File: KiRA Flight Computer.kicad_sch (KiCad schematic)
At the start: 44 parts, among them J1 Conn_01x04_Pin, J2 USB_C_Receptacle_USB2.0_14P, SW1 SW_Push, SW2 SW_SPDT, U1 ICM-426788P, U2 STM32F407VGTx, U3 MMC5883MA, U4 DPS368, U6 Wio-SX1262, U7 USBLC6-2P6, Y1 16MHz 7pF, Y2 OV_7604

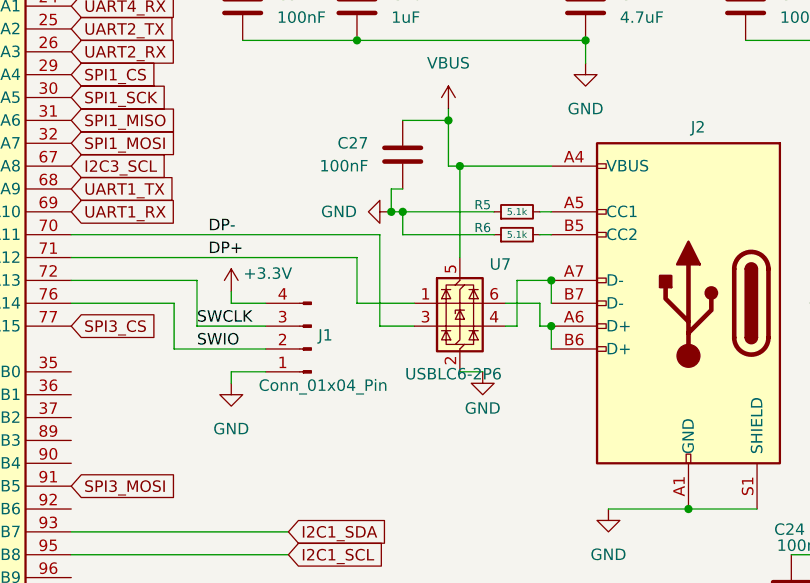
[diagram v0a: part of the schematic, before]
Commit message: Update PCB
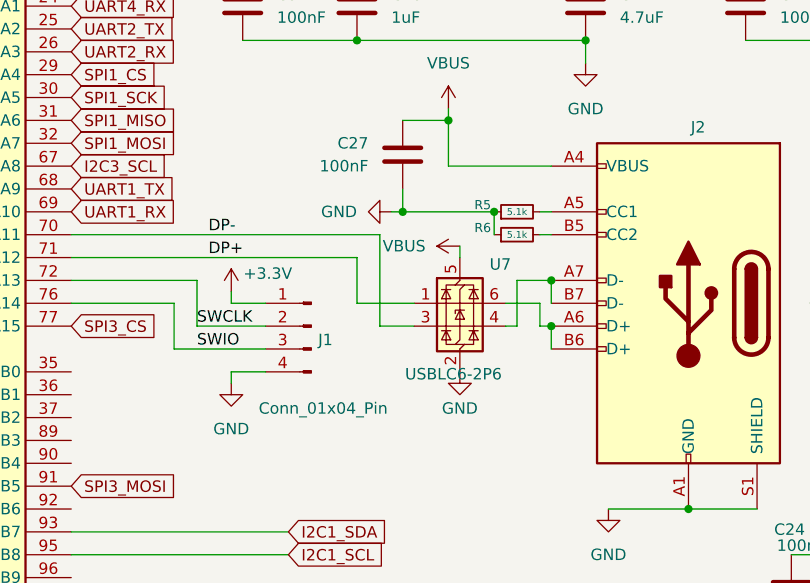
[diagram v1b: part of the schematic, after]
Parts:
- SW1: footprint Button_Switch_SMD:SW_Push_1P1T_NO_CK_PTS125Sx43PSMTR -> Button_Switch_SMD:SW_Push_1P1T_NO_CK_KSC6xxJ
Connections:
- net +3.3V: now also J1.1 (Pin_1); no longer J1.4 (Pin_4)
- net GND: now also J1.4 (Pin_4); no longer J1.1 (Pin_1)
- net SWCLK: now also J1.2 (Pin_2); no longer J1.3 (Pin_3)
- net SWIO: now also J1.3 (Pin_3); no longer J1.2 (Pin_2)
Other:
- moved on the sheet: J1
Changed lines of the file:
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@@
 	(paper "A4")
 	(junction
-		(at 135.89 63.5)
+		(at 217.17 48.26)
 		(diameter 0)
 		(color 0 0 0 0)
 	)
 	(junction
-		(at 217.17 48.26)
+		(at 135.89 63.5)
 		(diameter 0)
 		(color 0 0 0 0)
@@
 	)
 	(junction
+		(at 146.05 63.5)
+		(diameter 0)
+		(color 0 0 0 0)
+	)
+	(junction
 		(at 143.51 27.94)
 		(diameter 0)
@@
 	)
 	(junction
-		(at 134.62 63.5)
-		(diameter 0)
-		(color 0 0 0 0)
-	)
-	(junction
 		(at 16.51 77.47)
 		(diameter 0)
@@
 	)
 	(junction
-		(at 142.24 58.42)
-		(diameter 0)
-		(color 0 0 0 0)
-	)
-	(junction
 		(at 212.09 105.41)
 		(diameter 0)
@@
 	(wire
 		(pts
-			(xy 142.24 81.28) (xy 144.78 81.28)
-		)
-		(stroke
-			(width 0)
-			(type default)
-		)
-	)
-	(wire
-		(pts
 			(xy 156.21 20.32) (xy 168.91 20.32)
 		)
@@
 	(wire
 		(pts
-			(xy 135.89 66.04) (xy 135.89 63.5)
+			(xy 146.05 66.04) (xy 146.05 63.5)
 		)
 		(stroke
@@
 	(wire
 		(pts
-			(xy 146.05 66.04) (xy 135.89 66.04)
-		)
-		(stroke
-			(width 0)
-			(type default)
-		)
-	)
-	(wire
-		(pts
 			(xy 195.58 101.6) (xy 195.58 106.68)
 		)
@@
 	(wire
 		(pts
-			(xy 134.62 63.5) (xy 135.89 63.5)
-		)
-		(stroke
-			(width 0)
-			(type default)
-		)
-	)
-	(wire
-		(pts
 			(xy 259.08 128.27) (xy 259.08 134.62)
 		)
@@
 	(wire
 		(pts
+			(xy 135.89 63.5) (xy 146.05 63.5)
+		)
+		(stroke
+			(width 0)
+			(type default)
+		)
+	)
+	(wire
+		(pts
 			(xy 78.74 25.4) (xy 78.74 27.94)
 		)
@@
 	(wire
 		(pts
-			(xy 135.89 60.96) (xy 134.62 60.96)
-		)
-		(stroke
-			(width 0)
-			(type default)
-		)
-	)
-	(wire
-		(pts
-			(xy 142.24 58.42) (xy 152.4 58.42)
-		)
-		(stroke
-			(width 0)
-			(type default)
-		)
-	)
-	(wire
-		(pts
 			(xy 99.06 68.58) (xy 130.81 68.58)
 		)
@@
 	(wire
 		(pts
-			(xy 140.97 58.42) (xy 142.24 58.42)
+			(xy 140.97 58.42) (xy 152.4 58.42)
 		)
 		(stroke
@@
 	(wire
 		(pts
-			(xy 193.04 109.22) (xy 193.04 106.68)
+			(xy 135.89 63.5) (xy 134.62 63.5)
 		)
 		(stroke
@@
 	(wire
 		(pts
-			(xy 135.89 132.08) (xy 133.35 132.08)
+			(xy 193.04 109.22) (xy 193.04 106.68)
 		)
 		(stroke
@@
 	(wire
 		(pts
-			(xy 19.05 35.56) (xy 19.05 38.1)
+			(xy 135.89 132.08) (xy 133.35 132.08)
 		)
 		(stroke
@@
 	(wire
 		(pts
-			(xy 21.59 71.12) (xy 21.59 85.09)
+			(xy 19.05 35.56) (xy 19.05 38.1)
 		)
 		(stroke
@@
 	(wire
 		(pts
-			(xy 130.81 20.32) (xy 143.51 20.32)
+			(xy 21.59 71.12) (xy 21.59 85.09)
 		)
 		(stroke
@@
 	(wire
 		(pts
-			(xy 38.1 77.47) (xy 31.75 77.47)
+			(xy 130.81 20.32) (xy 143.51 20.32)
 		)
 		(stroke
@@
 	(wire
 		(pts
-			(xy 156.21 35.56) (xy 156.21 36.83)
+			(xy 38.1 77.47) (xy 31.75 77.47)
 		)
 		(stroke
@@
 	(wire
 		(pts
-			(xy 219.71 127) (xy 212.09 127)
+			(xy 156.21 35.56) (xy 156.21 36.83)
 		)
 		(stroke
@@
 	(wire
 		(pts
-			(xy 135.89 63.5) (xy 146.05 63.5)
+			(xy 219.71 127) (xy 212.09 127)
 		)
 		(stroke
@@
 	(wire
 		(pts
-			(xy 142.24 58.42) (xy 142.24 68.58)
-		)
-		(stroke
-			(width 0)
-			(type default)
-		)
-	)
-	(wire
-		(pts
 			(xy 133.35 66.04) (xy 133.35 76.2)
 		)
@@
 	(wire
 		(pts
-			(xy 134.62 60.96) (xy 134.62 63.5)
+			(xy 135.89 60.96) (xy 135.89 63.5)
 		)
 		(stroke
@@
 	(wire
 		(pts
+			(xy 142.24 67.31) (xy 142.24 68.58)
+		)
+		(stroke
+			(width 0)
+			(type default)
+		)
+	)
+	(wire
+		(pts
 			(xy 71.12 25.4) (xy 71.12 27.94)
 		)
@@
 			)
 		)
-		(property "Footprint" "Button_Switch_SMD:SW_Push_1P1T_NO_CK_PTS125Sx43PSMTR"
+		(property "Footprint" "Button_Switch_SMD:SW_Push_1P1T_NO_CK_KSC6xxJ"
 			(at 27.94 26.67 0)
 			(effects
@@
 	(symbol
 		(lib_id "power:GND")
-		(at 144.78 81.28 0)
+		(at 142.24 81.28 0)
 		(unit 1)
 		(exclude_from_sim no)
@@
 		(dnp no)
 		(property "Reference" "#PWR042"
-			(at 144.78 87.63 0)
+			(at 142.24 87.63 0)
 			(effects
 				(font
@@
 		)
 		(property "Value" "GND"
-			(at 144.78 85.344 0)
+			(at 142.24 85.344 0)
 			(effects
 				(font
@@
 		)
 		(property "Footprint" ""
-			(at 144.78 81.28 0)
+			(at 142.24 81.28 0)
 			(effects
 				(font
@@
 		)
 		(property "Datasheet" ""
-			(at 144.78 81.28 0)
+			(at 142.24 81.28 0)
 			(effects
 				(font
@@
 		)
 		(property "Description" "Power symbol creates a global label with name \"GND\" , ground"
-			(at 144.78 81.28 0)
+			(at 142.24 81.28 0)
 			(effects
 				(font
@@
 	(symbol
 		(lib_id "Connector:Conn_01x04_Pin")
-		(at 125.73 78.74 180)
+		(at 125.73 76.2 0)
+		(mirror y)
 		(unit 1)
 		(exclude_from_sim no)
@@
 		(dnp no)
 		(property "Reference" "J1"
-			(at 126.492 77.216 0)
+			(at 126.492 77.724 0)
 			(effects
 				(font
@@
 		)
 		(property "Value" "Conn_01x04_Pin"
-			(at 119.888 82.804 0)
+			(at 119.888 85.344 0)
 			(effects
 				(font
@@
 		)
 		(property "Footprint" "Connector_PinHeader_2.54mm:PinHeader_1x04_P2.54mm_Vertical"
-			(at 125.73 78.74 0)
+			(at 125.73 76.2 0)
 			(effects
 				(font
@@
 		)
 		(property "Datasheet" "~"
-			(at 125.73 78.74 0)
+			(at 125.73 76.2 0)
 			(effects
 				(font
@@
 		)
 		(property "Description" "Generic connector, single row, 01x04, script generated"
-			(at 125.73 78.74 0)
+			(at 125.73 76.2 0)
 			(effects
 				(font
@@
 	)
 	(symbol
+		(lib_id "power:VBUS")
+		(at 142.24 67.31 90)
+		(unit 1)
+		(exclude_from_sim no)
+		(in_bom yes)
+		(on_board yes)
+		(dnp no)
+		(fields_autoplaced yes)
+		(property "Reference" "#PWR073"
+			(at 146.05 67.31 0)
+			(effects
+				(font
+					(size 1.27 1.27)
+				)
+				(hide yes)
+			)
+		)
+		(property "Value" "VBUS"
+			(at 138.43 67.3099 90)
+			(effects
+				(font
+					(size 1.27 1.27)
+				)
+				(justify left)
+			)
+		)
+		(property "Footprint" ""
+			(at 142.24 67.31 0)
+			(effects
+				(font
+					(size 1.27 1.27)
+				)
+				(hide yes)
+			)
+		)
+		(property "Datasheet" ""
+			(at 142.24 67.31 0)
+			(effects
+				(font
+					(size 1.27 1.27)
+				)
+				(hide yes)
+			)
+		)
+		(property "Description" "Power symbol creates a global label with name \"VBUS\""
+			(at 142.24 67.31 0)
+			(effects
+				(font
+					(size 1.27 1.27)
+				)
+				(hide yes)
+			)
+		)
+		(pin "1"
+		)
+		(instances
+			(project "KiRA Flight Computer"
+				(path "/aff8106b-a9b7-4e48-85ad-25b2eb3ce379"
+					(reference "#PWR073")
+					(unit 1)
+				)
+			)
+		)
+	)
+	(symbol
 		(lib_id "power:GND")
 		(at 158.75 96.52 0)
@@
 		(on_board yes)
 		(dnp no)
-		(fields_autoplaced yes)
 		(property "Reference" "SW2"
 			(at 27.94 43.18 0)
@@
 					(reference "SW2")
 					(unit 1)
+				)
+				(path "/aff8106b-a9b7-4e48-85ad-25b2eb3ce379/ba160f04-df44-4adc-a5a3-9beb293319f2"
+					(reference "SW2")
+					(unit 1)

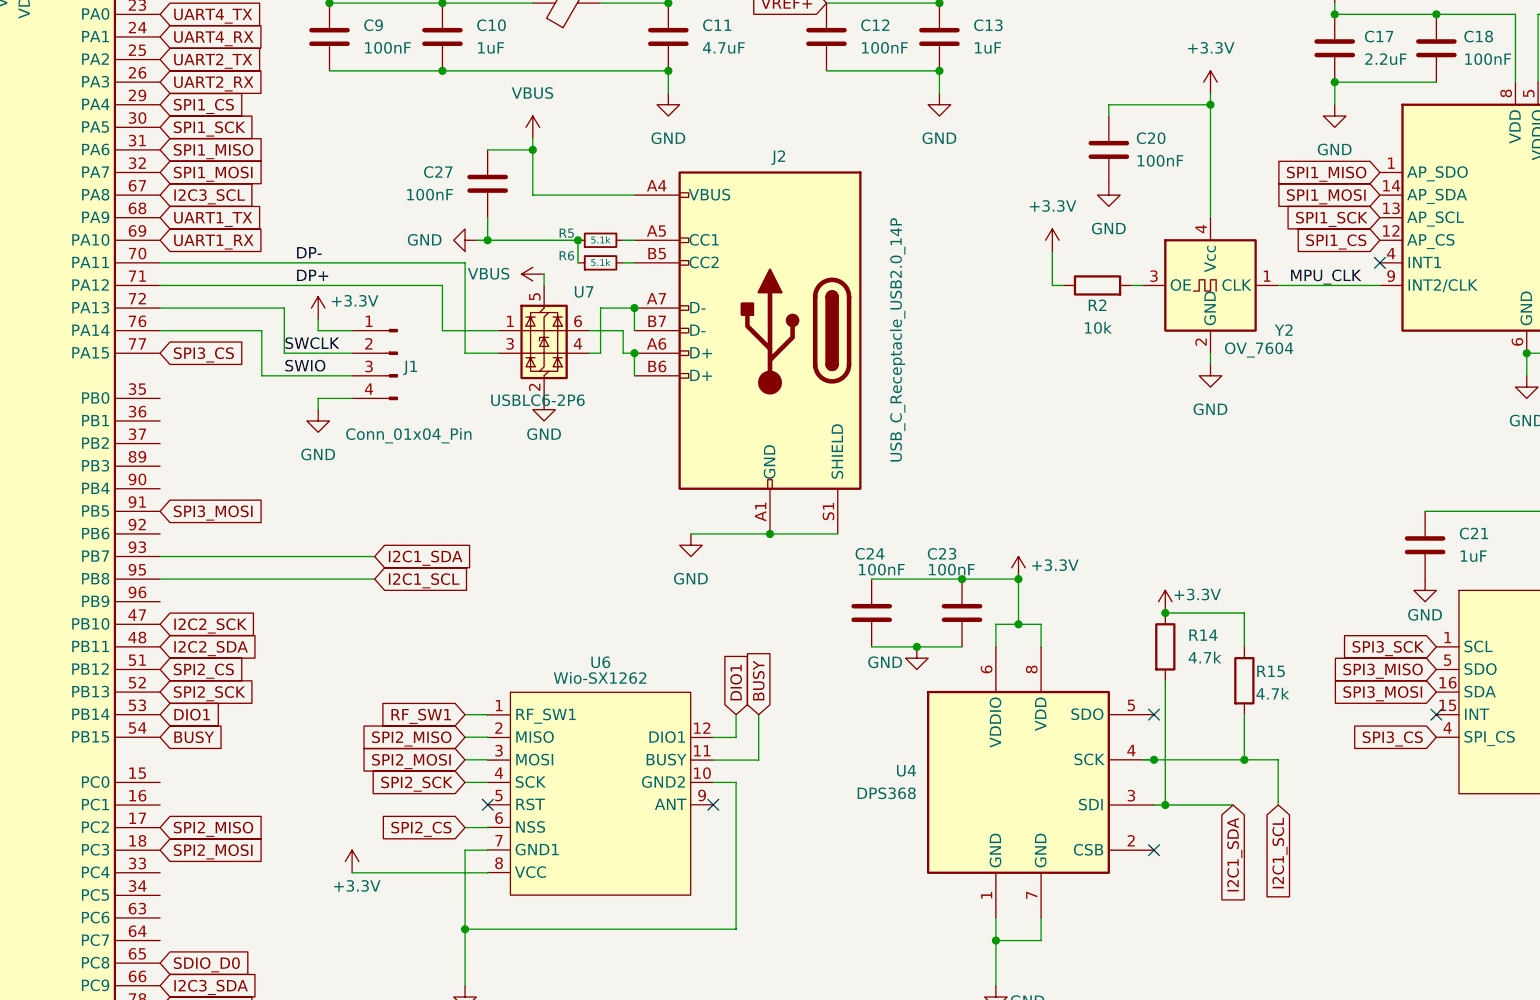
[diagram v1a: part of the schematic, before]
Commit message: Update PCB
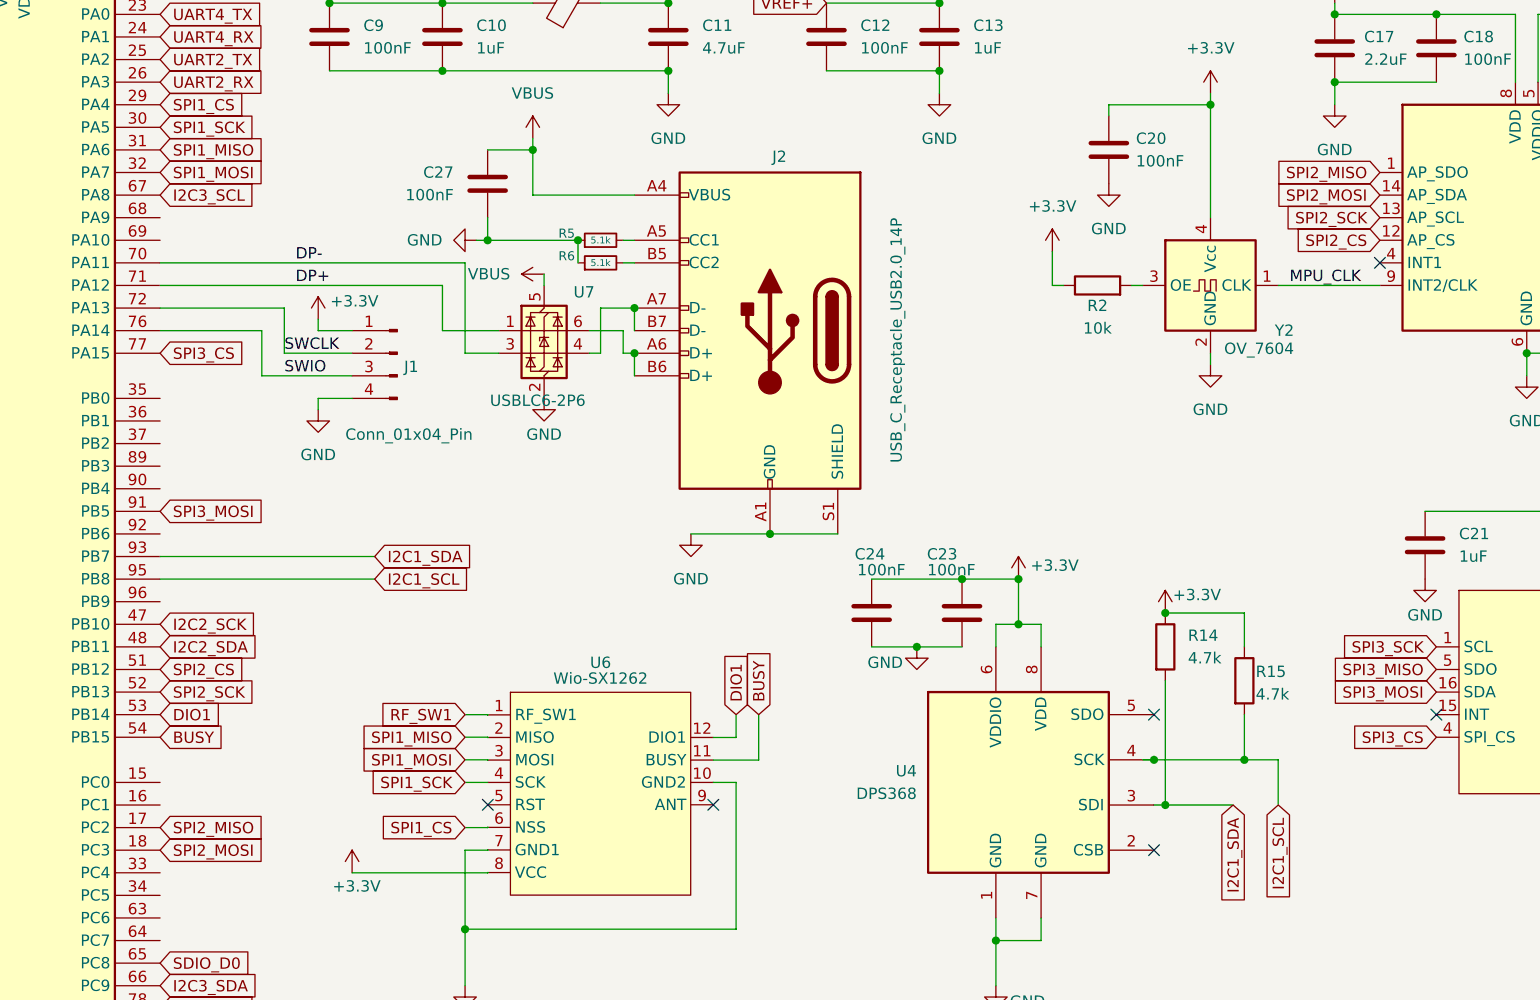
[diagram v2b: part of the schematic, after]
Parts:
- C19: footprint Capacitor_SMD:C_0402_1005Metric -> Capacitor_SMD:C_0603_1608Metric
- R1, R2: footprint Resistor_SMD:R_0402_1005Metric -> Resistor_SMD:R_0603_1608Metric
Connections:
- net SPI1_CS: now also U6.6 (NSS); no longer U1.12 (AP_CS)
- net SPI1_MISO: now also U6.2 (MISO); no longer U1.1 (AP_SDO)
- net SPI1_MOSI: now also U6.3 (MOSI); no longer U1.14 (AP_SDA)
- net SPI1_SCK: now also U6.4 (SCK); no longer U1.13 (AP_SCL)
- net SPI2_CS: now also U1.12 (AP_CS); no longer U6.6 (NSS)
- net SPI2_MISO: now also U1.1 (AP_SDO); no longer U6.2 (MISO)
- net SPI2_MOSI: now also U1.14 (AP_SDA); no longer U6.3 (MOSI)
- net SPI2_SCK: now also U1.13 (AP_SCL); no longer U6.4 (SCK)
- net UART1_RX: no longer names the net of U2.69 (PA10)
- net UART1_TX: no longer names the net of U2.68 (PA9)
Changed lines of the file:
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@@
 	(global_label "SPI1_MOSI"
 		(shape input)
-		(at 236.22 58.42 180)
+		(at 133.35 121.92 180)
 		(fields_autoplaced yes)
 		(effects
@@
 		)
 		(property "Intersheetrefs" "${INTERSHEET_REFS}"
-			(at 223.3772 58.42 0)
+			(at 120.5072 121.92 0)
 			(effects
 				(font
@@
 	(global_label "SPI2_SCK"
 		(shape input)
-		(at 133.35 124.46 180)
+		(at 236.22 60.96 180)
 		(fields_autoplaced yes)
 		(effects
@@
 		)
 		(property "Intersheetrefs" "${INTERSHEET_REFS}"
-			(at 121.3539 124.46 0)
+			(at 224.2239 60.96 0)
 			(effects
 				(font
@@
 	(global_label "SPI1_MISO"
 		(shape input)
-		(at 236.22 55.88 180)
+		(at 133.35 119.38 180)
 		(fields_autoplaced yes)
 		(effects
@@
 		)
 		(property "Intersheetrefs" "${INTERSHEET_REFS}"
-			(at 223.3772 55.88 0)
+			(at 120.5072 119.38 0)
 			(effects
 				(font
@@
 	(global_label "SPI2_CS"
 		(shape input)
-		(at 133.35 129.54 180)
+		(at 236.22 63.5 180)
 		(fields_autoplaced yes)
 		(effects
@@
 		)
 		(property "Intersheetrefs" "${INTERSHEET_REFS}"
-			(at 122.6239 129.54 0)
+			(at 225.4939 63.5 0)
 			(effects
 				(font
@@
 		)
 	)
-	(global_label "UART1_TX"
-		(shape input)
-		(at 99.06 60.96 0)
-		(fields_autoplaced yes)
-		(effects
-			(font
-				(size 1.27 1.27)
-			)
-			(justify left)
-		)
-		(property "Intersheetrefs" "${INTERSHEET_REFS}"
-			(at 111.0561 60.96 0)
-			(effects
-				(font
-					(size 1.27 1.27)
-				)
-				(justify left)
-				(hide yes)
-			)
-		)
-	)
 	(global_label "I2C2_SDA"
 		(shape input)
@@
 		)
 	)
-	(global_label "UART1_RX"
-		(shape input)
-		(at 99.06 63.5 0)
-		(fields_autoplaced yes)
-		(effects
-			(font
-				(size 1.27 1.27)
-			)
-			(justify left)
-		)
-		(property "Intersheetrefs" "${INTERSHEET_REFS}"
-			(at 111.3585 63.5 0)
-			(effects
-				(font
-					(size 1.27 1.27)
-				)
-				(justify left)
-				(hide yes)
-			)
-		)
-	)
 	(global_label "UART2_TX"
 		(shape input)
@@
 	(global_label "SPI2_MISO"
 		(shape input)
-		(at 133.35 119.38 180)
+		(at 236.22 55.88 180)
 		(fields_autoplaced yes)
 		(effects
@@
 		)
 		(property "Intersheetrefs" "${INTERSHEET_REFS}"
-			(at 120.5072 119.38 0)
+			(at 223.3772 55.88 0)
 			(effects
 				(font
@@
 	(global_label "SPI2_MOSI"
 		(shape input)
-		(at 133.35 121.92 180)
+		(at 236.22 58.42 180)
 		(fields_autoplaced yes)
 		(effects
@@
 		)
 		(property "Intersheetrefs" "${INTERSHEET_REFS}"
-			(at 120.5072 121.92 0)
+			(at 223.3772 58.42 0)
 			(effects
 				(font
@@
 	(global_label "SPI1_SCK"
 		(shape input)
-		(at 236.22 60.96 180)
+		(at 133.35 124.46 180)
 		(fields_autoplaced yes)
 		(effects
@@
 		)
 		(property "Intersheetrefs" "${INTERSHEET_REFS}"
-			(at 224.2239 60.96 0)
+			(at 121.3539 124.46 0)
 			(effects
 				(font
@@
 	(global_label "SPI1_CS"
 		(shape input)
-		(at 236.22 63.5 180)
+		(at 133.35 129.54 180)
 		(fields_autoplaced yes)
 		(effects
@@
 		)
 		(property "Intersheetrefs" "${INTERSHEET_REFS}"
-			(at 225.4939 63.5 0)
+			(at 122.6239 129.54 0)
 			(effects
 				(font
@@
 			)
 		)
-		(property "Footprint" "Capacitor_SMD:C_0402_1005Metric"
+		(property "Footprint" "Capacitor_SMD:C_0603_1608Metric"
 			(at 272.7452 45.72 0)
 			(effects
@@
 			)
 		)
-		(property "Footprint" "Resistor_SMD:R_0402_1005Metric"
+		(property "Footprint" "Resistor_SMD:R_0603_1608Metric"
 			(at 204.47 70.358 90)
 			(effects
@@
 			)
 		)
-		(property "Footprint" "Resistor_SMD:R_0402_1005Metric"
+		(property "Footprint" "Resistor_SMD:R_0603_1608Metric"
 			(at 41.91 47.498 90)
 			(effects
